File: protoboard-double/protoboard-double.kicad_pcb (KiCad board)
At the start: 2 copper layers, 50.8 x 58.4 mm, 23 parts, among them J1 MODULE_HEADER, J2 MODULE_HEADER, P1 CONN_01X22, P10 CONN_01X22, P11 CONN_01X22, P12 CONN_01X22, P13 CONN_01X22, P14 CONN_01X22, P15 CONN_01X22, P16 CONN_01X22, P17 CONN_01X22, P18 CONN_01X22, P19 CONN_01X22, P2 CONN_01X22, P3 CONN_01X22, P4 CONN_01X22, P5 CONN_01X22, P6 CONN_01X22, P7 CONN_01X22, P8 CONN_01X22, P9 CONN_01X22

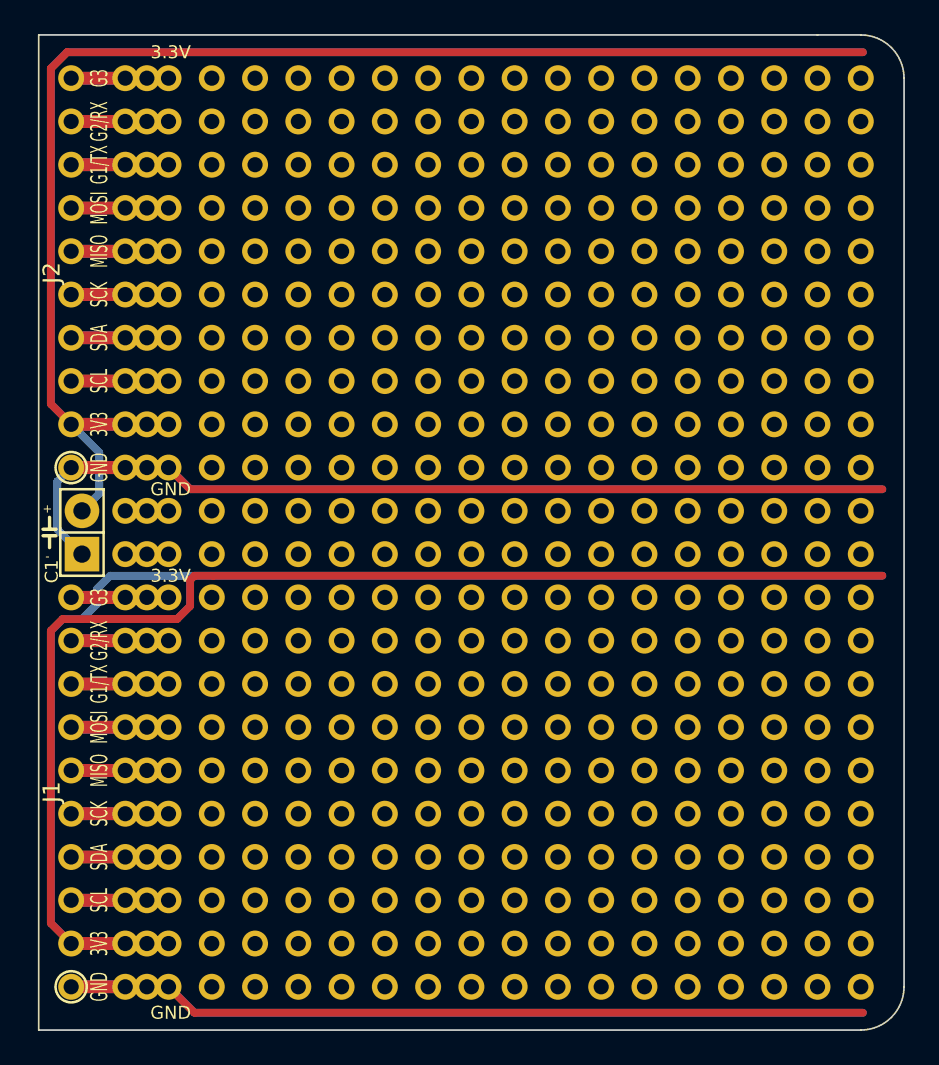
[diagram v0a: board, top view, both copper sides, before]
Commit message: feedback incorporated for doublewide. all aboard the PCB ship!
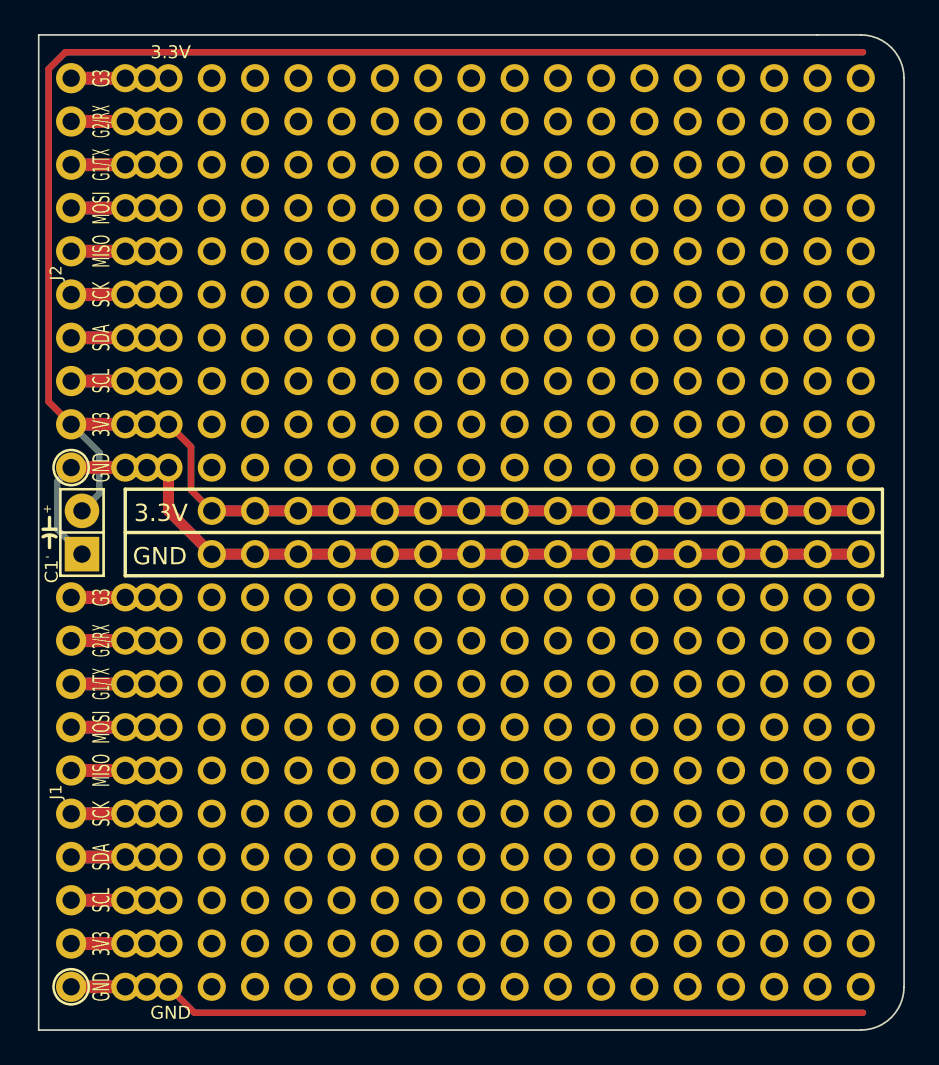
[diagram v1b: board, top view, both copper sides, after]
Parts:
- added P20: CONN_01X10, parts:1x10_BIG, F.Cu at (106.7, 82.5)
- added P21: CONN_01X10, parts:1x10_BIG, F.Cu at (108.0, 113.0)
- added P22: CONN_01X10, parts:1x10_BIG, F.Cu at (108.0, 82.5)
- J1, J2: footprint parts:MODULE_HEADER_MODULE -> parts:MODULE_HEADER_MODULE_BIG
- P1, P10, P11, P12, P13, P14, P15, P16, P17, P18, P19, P2, P4, P5, P7, P8: footprint parts:1x22 -> parts:1x22_BIG
- P3, P6, P9: value CONN_01X22 -> CONN_01X10; footprint parts:1x22 -> parts:1x10_BIG
- SILK1: footprint parts:TESSEL-HEXAGON-LOGO-BACK -> parts:TESSEL-HEXAGON-LOGO-BACK-BIG
- moved P6 15.3 mm to (109.2, 82.5)
- moved P3 15.2 mm to (109.2, 113.0)
- moved P9 15.2 mm to (106.7, 113.0)
- moved SILK1 8.25 mm to (127.0, 97.8)
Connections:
- P1 pad 11: Net-(P1-Pad11) -> Net-(C1-Pad1)
- P1 pad 12: Net-(P1-Pad12) -> Net-(C1-Pad2)
- P10 pad 11: Net-(P10-Pad11) -> Net-(C1-Pad1)
- P10 pad 12: Net-(P10-Pad12) -> Net-(C1-Pad2)
- P11 pad 11: Net-(P11-Pad11) -> Net-(C1-Pad1)
- P11 pad 12: Net-(P11-Pad12) -> Net-(C1-Pad2)
- P12 pad 11: Net-(P12-Pad11) -> Net-(C1-Pad1)
- P12 pad 12: Net-(P12-Pad12) -> Net-(C1-Pad2)
- P13 pad 11: Net-(P13-Pad11) -> Net-(C1-Pad1)
- P13 pad 12: Net-(P13-Pad12) -> Net-(C1-Pad2)
- P14 pad 11: Net-(P14-Pad11) -> Net-(C1-Pad1)
- P14 pad 12: Net-(P14-Pad12) -> Net-(C1-Pad2)
- P15 pad 11: Net-(P15-Pad11) -> Net-(C1-Pad1)
- P15 pad 12: Net-(P15-Pad12) -> Net-(C1-Pad2)
- P16 pad 11: Net-(P16-Pad11) -> Net-(C1-Pad1)
- P16 pad 12: Net-(P16-Pad12) -> Net-(C1-Pad2)
- P17 pad 11: Net-(P17-Pad11) -> Net-(C1-Pad1)
- P17 pad 12: Net-(P17-Pad12) -> Net-(C1-Pad2)
- P18 pad 11: Net-(P18-Pad11) -> Net-(C1-Pad1)
- P18 pad 12: Net-(P18-Pad12) -> Net-(C1-Pad2)
- P19 pad 11: Net-(P19-Pad11) -> Net-(C1-Pad1)
- P19 pad 12: Net-(P19-Pad12) -> Net-(C1-Pad2)
- P2 pad 11: Net-(P2-Pad11) -> Net-(C1-Pad1)
- P2 pad 12: Net-(P2-Pad12) -> Net-(C1-Pad2)
- P4 pad 11: Net-(P4-Pad11) -> Net-(C1-Pad1)
- P4 pad 12: Net-(P4-Pad12) -> Net-(C1-Pad2)
- P5 pad 11: Net-(P5-Pad11) -> Net-(C1-Pad1)
- P5 pad 12: Net-(P5-Pad12) -> Net-(C1-Pad2)
- P6 pad 1: Net-(J1-Pad1) -> Net-(C1-Pad1)
- P6 pad 10: Net-(J1-Pad10) -> Net-(J2-Pad10)
- P6 pad 2: Net-(J1-Pad2) -> Net-(C1-Pad2)
- P6 pad 3: Net-(J1-Pad3) -> Net-(J2-Pad3)
- P6 pad 4: Net-(J1-Pad4) -> Net-(J2-Pad4)
- P6 pad 5: Net-(J1-Pad5) -> Net-(J2-Pad5)
- P6 pad 6: Net-(J1-Pad6) -> Net-(J2-Pad6)
- P6 pad 7: Net-(J1-Pad7) -> Net-(J2-Pad7)
- P6 pad 8: Net-(J1-Pad8) -> Net-(J2-Pad8)
- P6 pad 9: Net-(J1-Pad9) -> Net-(J2-Pad9)
- P7 pad 11: Net-(P7-Pad11) -> Net-(C1-Pad1)
- P7 pad 12: Net-(P7-Pad12) -> Net-(C1-Pad2)
- P8 pad 11: Net-(P8-Pad11) -> Net-(C1-Pad1)
- P8 pad 12: Net-(P8-Pad12) -> Net-(C1-Pad2)
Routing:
- net Net-(J1-Pad2): track 145.1 -> 5.72 mm
- net Net-(C1-Pad2): track 157.2 -> 246.0 mm
- net Net-(P3-Pad12): track 3.81 -> 0.00 mm
- net Net-(C1-Pad1): track 99.1 -> 102.7 mm
- net Net-(P3-Pad11): track 2.54 -> 0.00 mm
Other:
- board text added: "diy- module"
- board text removed: "diy-module"
